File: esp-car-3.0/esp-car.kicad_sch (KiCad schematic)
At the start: 37 parts, among them J1 Conn_01x07_Socket, J2 Conn_01x07_Socket, U1 ESP32-DEVKIT-V1, U3 L293D

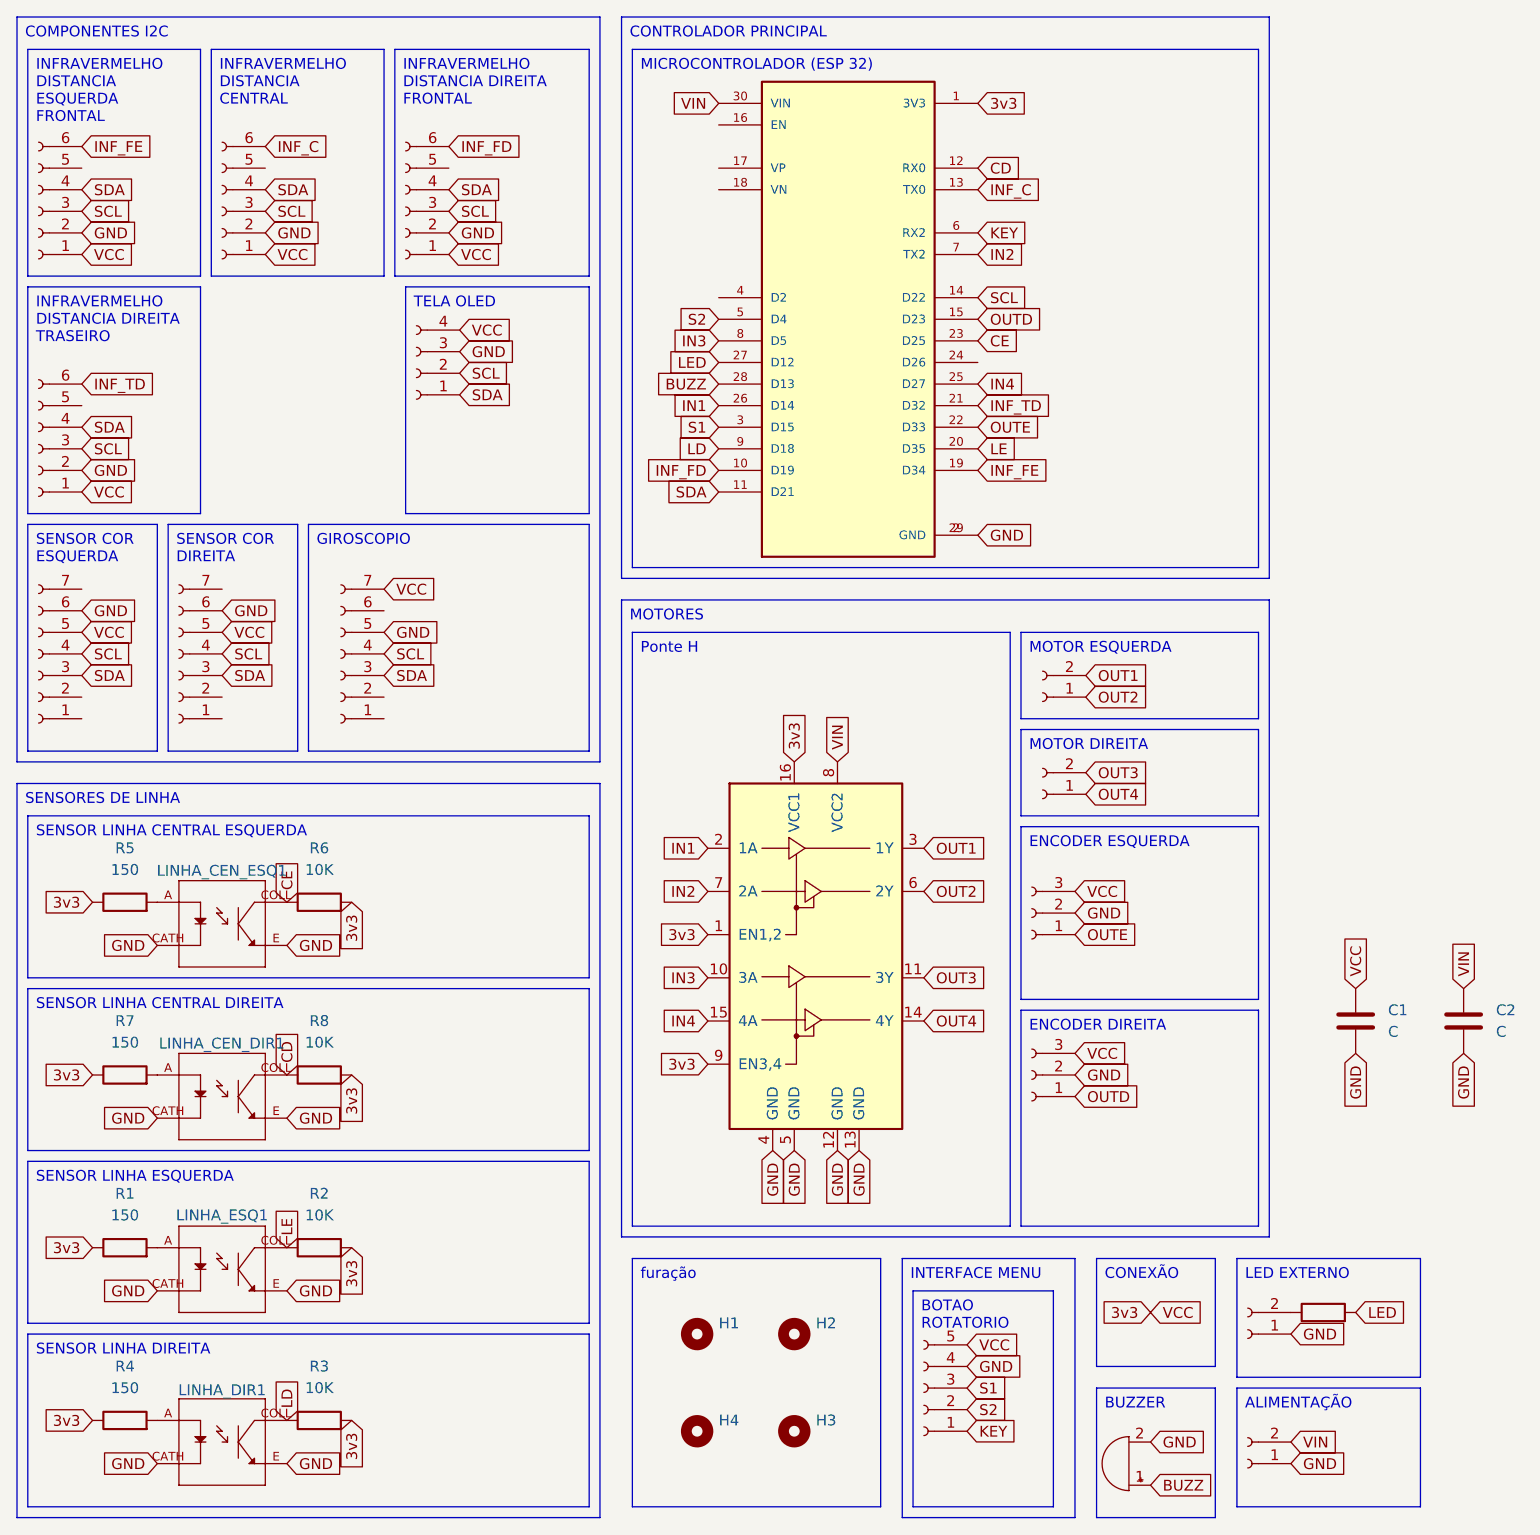
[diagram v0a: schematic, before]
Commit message: .
.
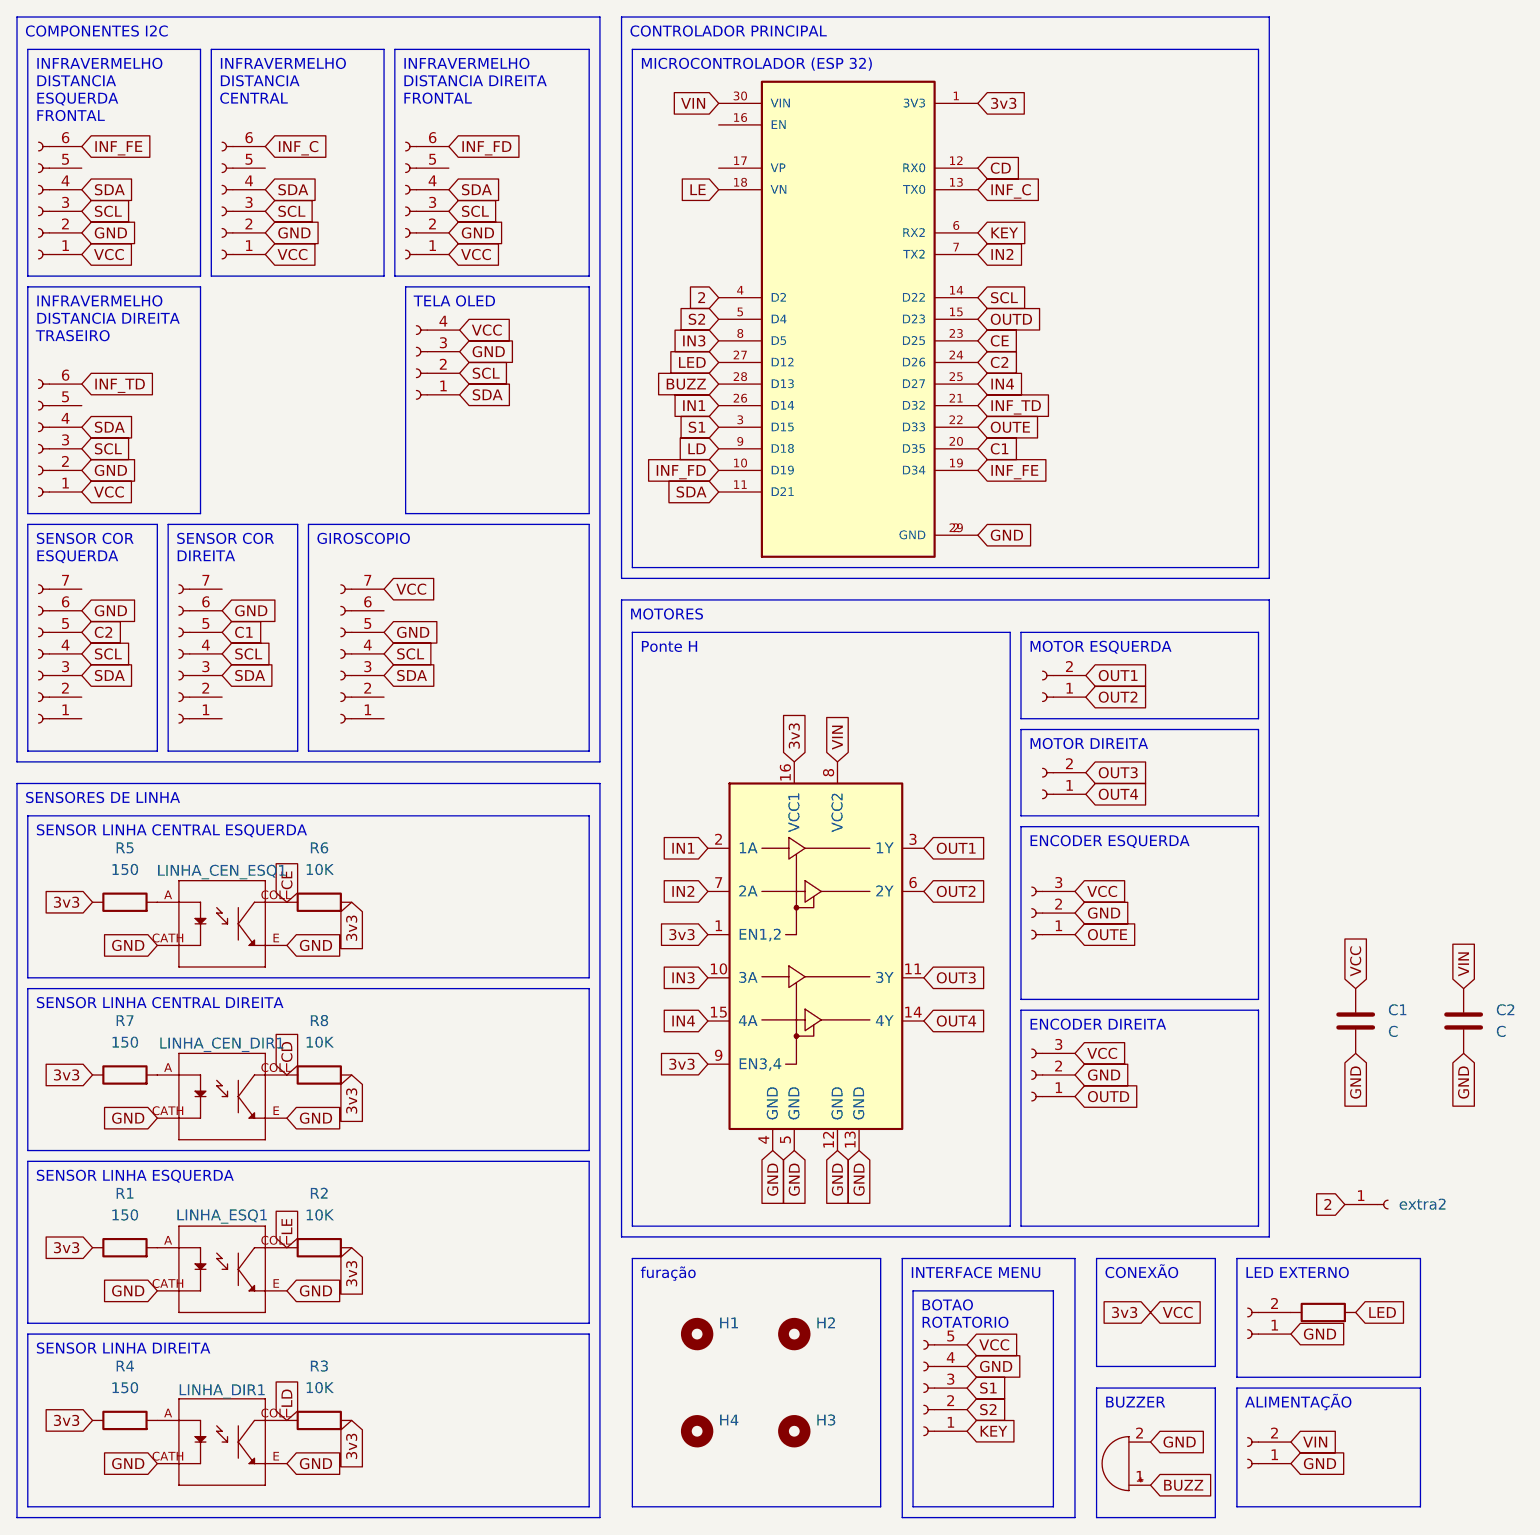
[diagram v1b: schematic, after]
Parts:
- added extra2: Conn_01x01_Socket, Connector_PinSocket_2.54mm:PinSocket_1x01_P2.54mm_Vertical, symbol Connector:Conn_01x01_Socket
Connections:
- net 3v3: no longer J1.5 (Pin_5), J2.5 (Pin_5)
- net LE: now also U1.18 (VN); no longer U1.20 (D35)
- net C2: now reaches U1.24 (D26)
- net C2: now also J2.5 (Pin_5)
- net 2: now reaches U1.4 (D2)
- net 2: now also extra2.1 (Pin_1)
- new net C1: J1.5 (Pin_5), U1.20 (D35)
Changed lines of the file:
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@@
 		)
 	)
-	(global_label "VCC"
-		(shape input)
-		(at 38.1 86.36 0)
-		(fields_autoplaced yes)
-		(effects
-			(font
-				(size 1.27 1.27)
-			)
-			(justify left)
-		)
-		(property "Intersheetrefs" "${INTERSHEET_REFS}"
-			(at 44.7138 86.36 0)
-			(effects
-				(font
-					(size 1.27 1.27)
-				)
-				(justify left)
-				(hide yes)
-			)
-		)
-	)
 	(global_label "GND"
 		(shape input)
@@
 		)
 	)
+	(global_label "C2"
+		(shape input)
+		(at 21.59 86.36 0)
+		(fields_autoplaced yes)
+		(effects
+			(font
+				(size 1.27 1.27)
+			)
+			(justify left)
+		)
+		(property "Intersheetrefs" "${INTERSHEET_REFS}"
+			(at 27.0547 86.36 0)
+			(effects
+				(font
+					(size 1.27 1.27)
+				)
+				(justify left)
+				(hide yes)
+			)
+		)
+	)
 	(global_label "GND"
 		(shape input)
@@
 	(global_label "LE"
 		(shape input)
-		(at 127 64.77 0)
+		(at 96.52 34.29 180)
 		(fields_autoplaced yes)
 		(effects
@@
 				(size 1.27 1.27)
 			)
-			(justify left)
+			(justify right)
 		)
 		(property "Intersheetrefs" "${INTERSHEET_REFS}"
-			(at 132.1623 64.77 0)
+			(at 91.3577 34.29 0)
 			(effects
 				(font
 					(size 1.27 1.27)
 				)
-				(justify left)
+				(justify right)
 				(hide yes)
 			)
@@
 		)
 	)
+	(global_label "C1"
+		(shape input)
+		(at 127 64.77 0)
+		(fields_autoplaced yes)
+		(effects
+			(font
+				(size 1.27 1.27)
+			)
+			(justify left)
+		)
+		(property "Intersheetrefs" "${INTERSHEET_REFS}"
+			(at 132.4647 64.77 0)
+			(effects
+				(font
+					(size 1.27 1.27)
+				)
+				(justify left)
+				(hide yes)
+			)
+		)
+	)
 	(global_label "S1"
 		(shape input)
@@
 		)
 	)
+	(global_label "2"
+		(shape input)
+		(at 96.52 46.99 180)
+		(fields_autoplaced yes)
+		(effects
+			(font
+				(size 1.27 1.27)
+			)
+			(justify right)
+		)
+		(property "Intersheetrefs" "${INTERSHEET_REFS}"
+			(at 92.3253 46.99 0)
+			(effects
+				(font
+					(size 1.27 1.27)
+				)
+				(justify right)
+				(hide yes)
+			)
+		)
+	)
 	(global_label "SDA"
 		(shape input)
@@
 		)
 	)
+	(global_label "C1"
+		(shape input)
+		(at 38.1 86.36 0)
+		(fields_autoplaced yes)
+		(effects
+			(font
+				(size 1.27 1.27)
+			)
+			(justify left)
+		)
+		(property "Intersheetrefs" "${INTERSHEET_REFS}"
+			(at 43.5647 86.36 0)
+			(effects
+				(font
+					(size 1.27 1.27)
+				)
+				(justify left)
+				(hide yes)
+			)
+		)
+	)
 	(global_label "OUT2"
 		(shape input)
@@
 		)
 	)
+	(global_label "2"
+		(shape input)
+		(at 170.18 153.67 180)
+		(fields_autoplaced yes)
+		(effects
+			(font
+				(size 1.27 1.27)
+			)
+			(justify right)
+		)
+		(property "Intersheetrefs" "${INTERSHEET_REFS}"
+			(at 165.9853 153.67 0)
+			(effects
+				(font
+					(size 1.27 1.27)
+				)
+				(justify right)
+				(hide yes)
+			)
+		)
+	)
 	(global_label "GND"
 		(shape input)
@@
 		)
 	)
-	(global_label "VCC"
-		(shape input)
-		(at 21.59 86.36 0)
-		(fields_autoplaced yes)
-		(effects
-			(font
-				(size 1.27 1.27)
-			)
-			(justify left)
-		)
-		(property "Intersheetrefs" "${INTERSHEET_REFS}"
-			(at 28.2038 86.36 0)
-			(effects
-				(font
-					(size 1.27 1.27)
-				)
-				(justify left)
-				(hide yes)
-			)
-		)
-	)
 	(global_label "GND"
 		(shape input)
@@
 		)
 	)
+	(global_label "C2"
+		(shape input)
+		(at 127 54.61 0)
+		(fields_autoplaced yes)
+		(effects
+			(font
+				(size 1.27 1.27)
+			)
+			(justify left)
+		)
+		(property "Intersheetrefs" "${INTERSHEET_REFS}"
+			(at 132.4647 54.61 0)
+			(effects
+				(font
+					(size 1.27 1.27)
+				)
+				(justify left)
+				(hide yes)
+			)
+		)
+	)
 	(global_label "OUTE"
 		(shape input)
@@
 					(unit 1)
 				)
+			)
+		)
+	)
+	(symbol
+		(lib_id "Connector:Conn_01x01_Socket")
+		(at 175.26 153.67 0)
+		(unit 1)
+		(exclude_from_sim no)
+		(in_bom yes)
+		(on_board yes)
+		(dnp no)
+		(fields_autoplaced yes)
+		(property "Reference" "extra2"
+			(at 176.53 153.6699 0)
+			(effects
+				(font
+					(size 1.27 1.27)
+				)
+				(justify left)
+			)
+		)
+		(property "Value" "Conn_01x01_Socket"
+			(at 176.53 154.9399 0)
+			(effects
+				(font
+					(size 1.27 1.27)
+				)
+				(justify left)
+				(hide yes)
+			)
+		)
+		(property "Footprint" "Connector_PinSocket_2.54mm:PinSocket_1x01_P2.54mm_Vertical"
+			(at 175.26 153.67 0)
+			(effects
+				(font
+					(size 1.27 1.27)
+				)
+				(hide yes)
+			)
+		)
+		(property "Datasheet" "~"
+			(at 175.26 153.67 0)
+			(effects
+				(font
+					(size 1.27 1.27)
+				)
+				(hide yes)
+			)
+		)
+		(property "Description" "Generic connector, single row, 01x01, script generated"
+			(at 175.26 153.67 0)
+			(effects
+				(font
+					(size 1.27 1.27)
+				)
+				(hide yes)
+			)
+		)
+		(pin "1"
+		)
+		(instances
+			(project "esp-car"
+				(path "/d21b542b-1246-4c6e-b3e1-1cc2382a01d2"
+					(reference "extra2")
+					(unit 1)
+				)

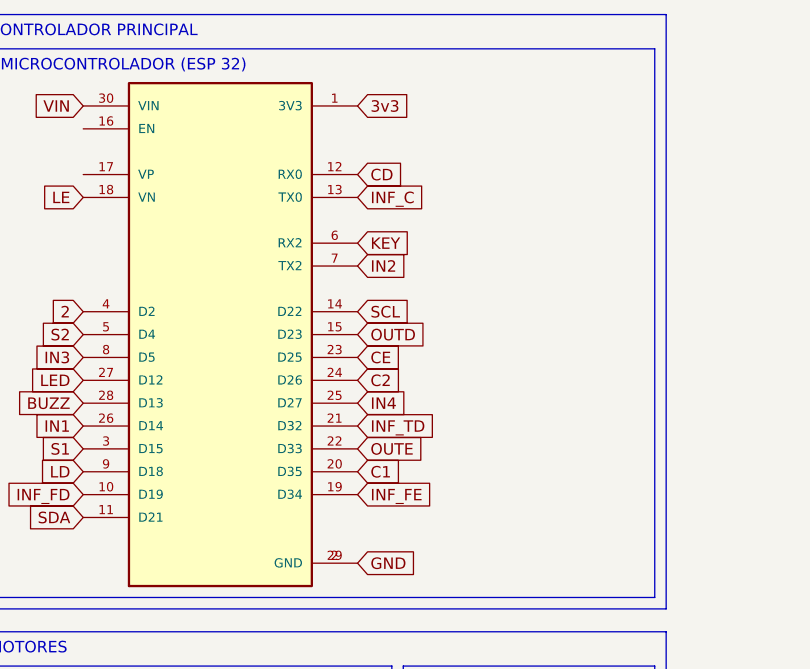
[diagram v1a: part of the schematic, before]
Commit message: espcar newvember
modelo quadradao
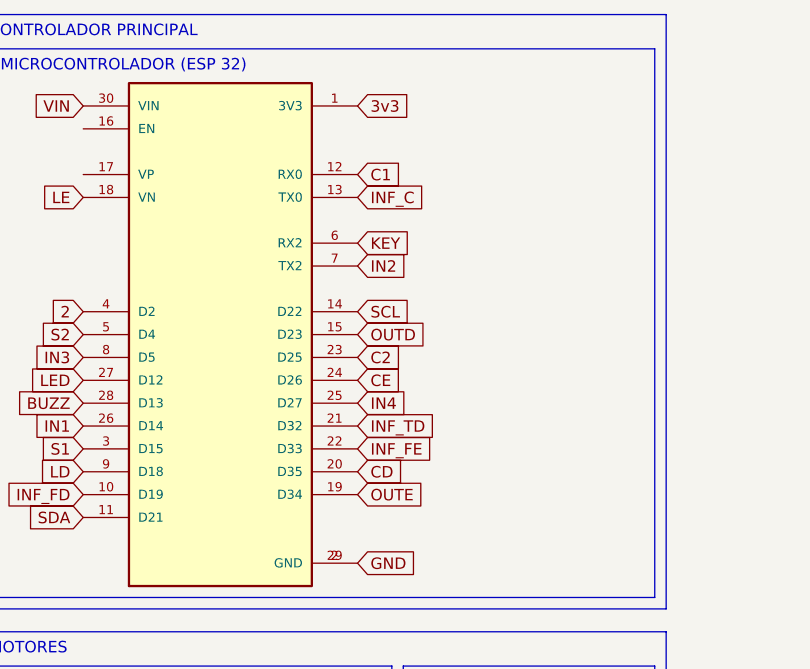
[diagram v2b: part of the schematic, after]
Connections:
- net C1: now also U1.12 (RX0); no longer U1.20 (D35)
- net C2: now also U1.23 (D25); no longer U1.24 (D26)
- net CD: now also U1.20 (D35); no longer U1.12 (RX0)
- net CE: now also U1.24 (D26); no longer U1.23 (D25)
- net INF_FE: now also U1.22 (D33); no longer U1.19 (D34)
- net OUTE: now also U1.19 (D34); no longer U1.22 (D33)
